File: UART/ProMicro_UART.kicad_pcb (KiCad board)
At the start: 2 copper layers, 17.8 x 33 mm, 56 parts, among them J2 Conn_01x06, J3 USB_B_Mini, U1 FT232H, U2 93CxxB, U3 AZ1117-3.3, Y1 12MHz

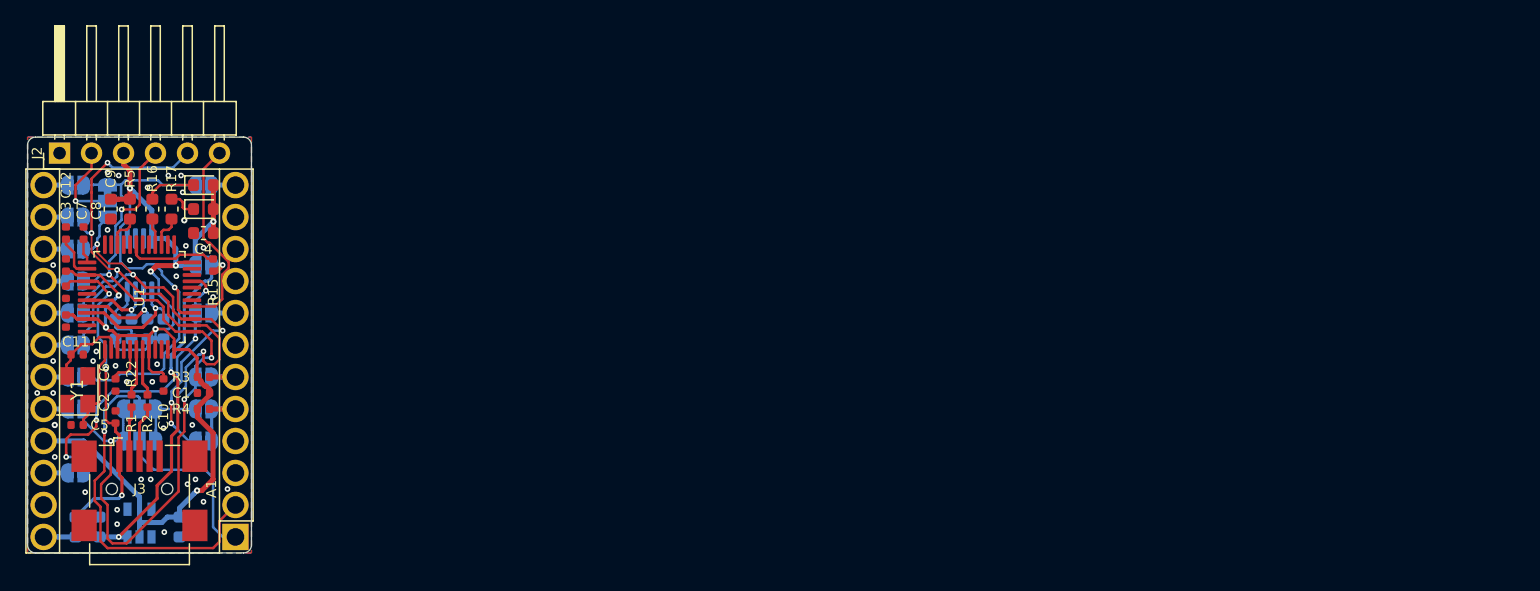
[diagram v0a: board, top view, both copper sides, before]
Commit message: UART
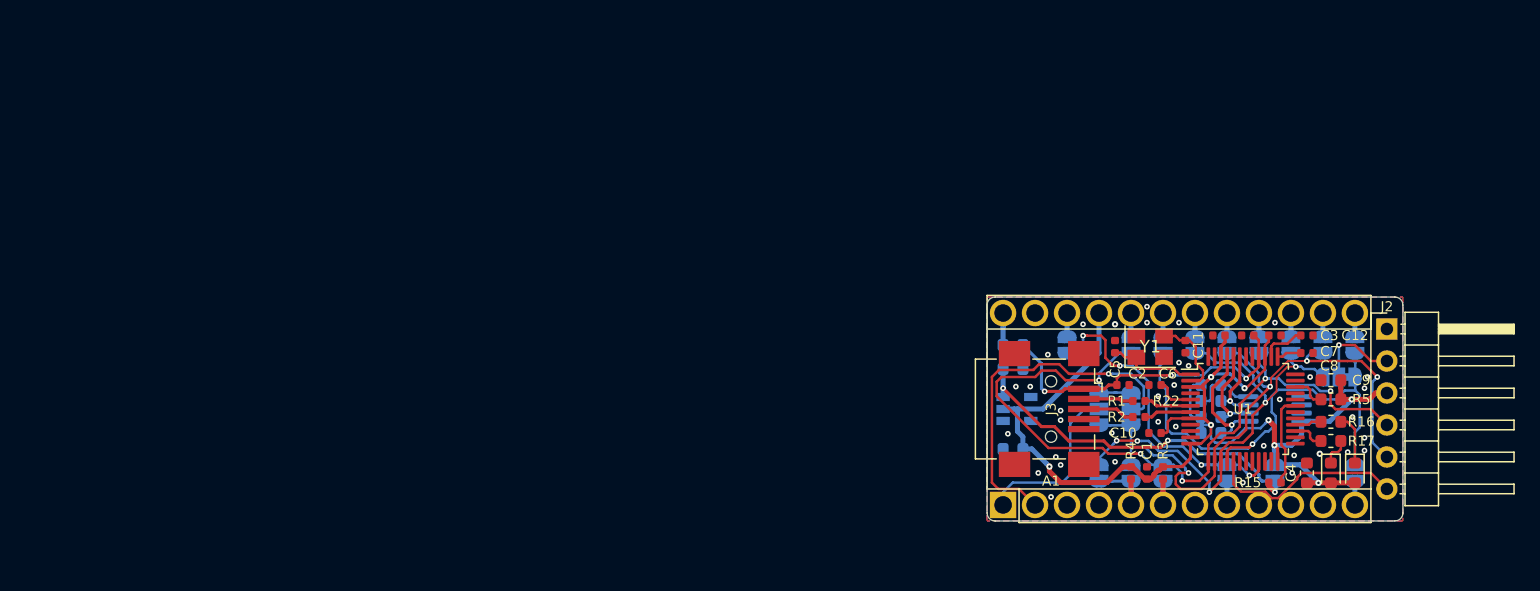
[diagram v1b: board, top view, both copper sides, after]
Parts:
- moved J2 106.3 mm to (157.5, 87.6), turned to 0 degrees
- moved JP5 102.4 mm to (154.9, 88.9), turned to 90 degrees
- moved JP2 99.6 mm to (152.4, 88.9), turned to 90 degrees
- moved C7 98.9 mm to (151.1, 88.1), turned to 0 degrees
- moved JP16 98.8 mm to (153.7, 91.4), turned to 180 degrees
- moved C9 97.8 mm to (153.0, 91.7), turned to 180 degrees
- moved C8 97.6 mm to (151.1, 89.5), turned to 0 degrees
- moved JP3 96.8 mm to (149.9, 88.9), turned to 90 degrees
- moved R5 96.6 mm to (153.0, 93.2), turned to 0 degrees
- moved C12 96.2 mm to (148.6, 88.1), turned to 0 degrees
- moved R16 95.1 mm to (153.0, 95.0), turned to 0 degrees
- moved D1 94.3 mm to (154.9, 99.1), turned to 270 degrees
- moved JP4 94.3 mm to (154.9, 99.1), turned to 270 degrees
- moved JP1 94.1 mm to (147.3, 88.9), turned to 90 degrees
- moved C3 93.9 mm to (146.4, 88.1), turned to 180 degrees
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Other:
- board size 17.8 x 33 mm -> 33 x 17.8 mm
